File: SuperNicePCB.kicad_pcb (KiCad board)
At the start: 4 copper layers, 75 x 85 mm, 66 parts, among them U1 ESP32-S3-WROOM-1-N8, U2 SY8089AAAC, U3 SGM2048-ADJXTEK8G/TR, U4 ICS-43434_C5656610, U5 AM312, U6 SCD40-D-R1, U7 SHT40-AD1B-R3, U8 HLK-LD6002, U9 DWM3000TR13

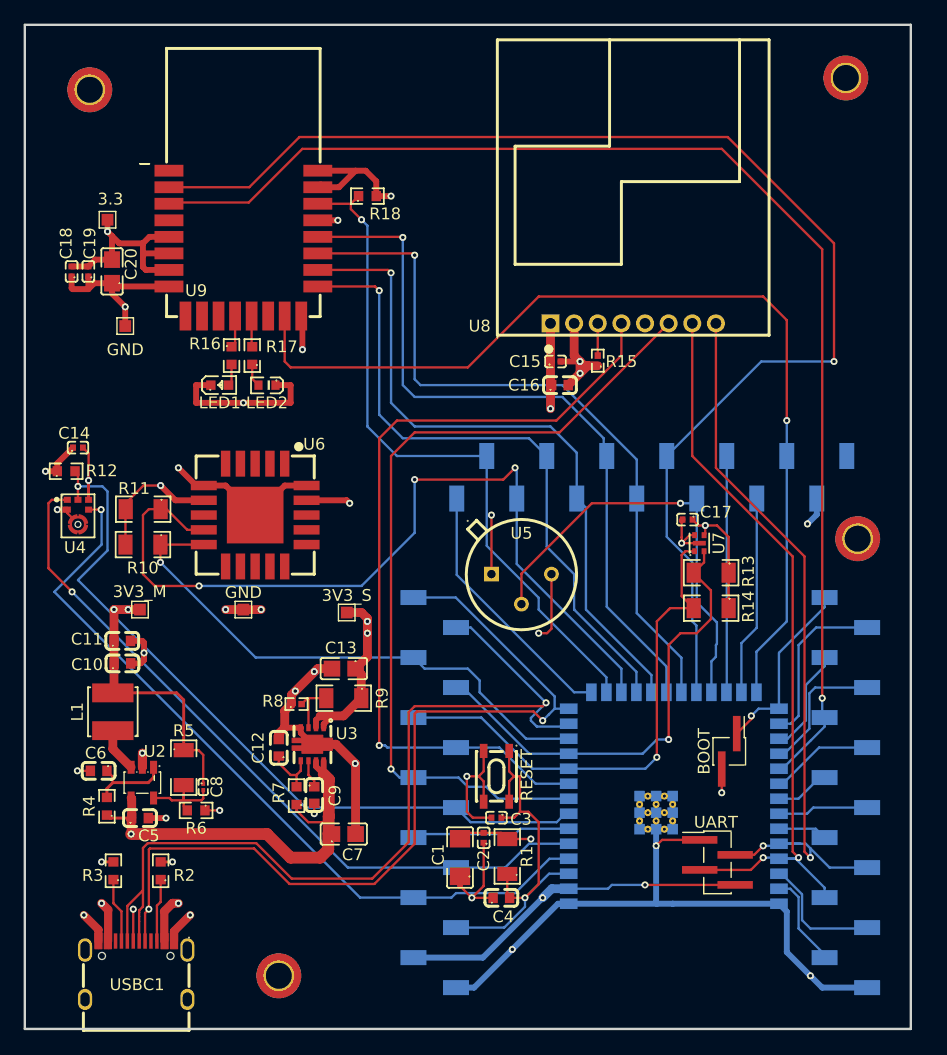
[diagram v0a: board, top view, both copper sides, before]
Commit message: Label + test commit Mathieu
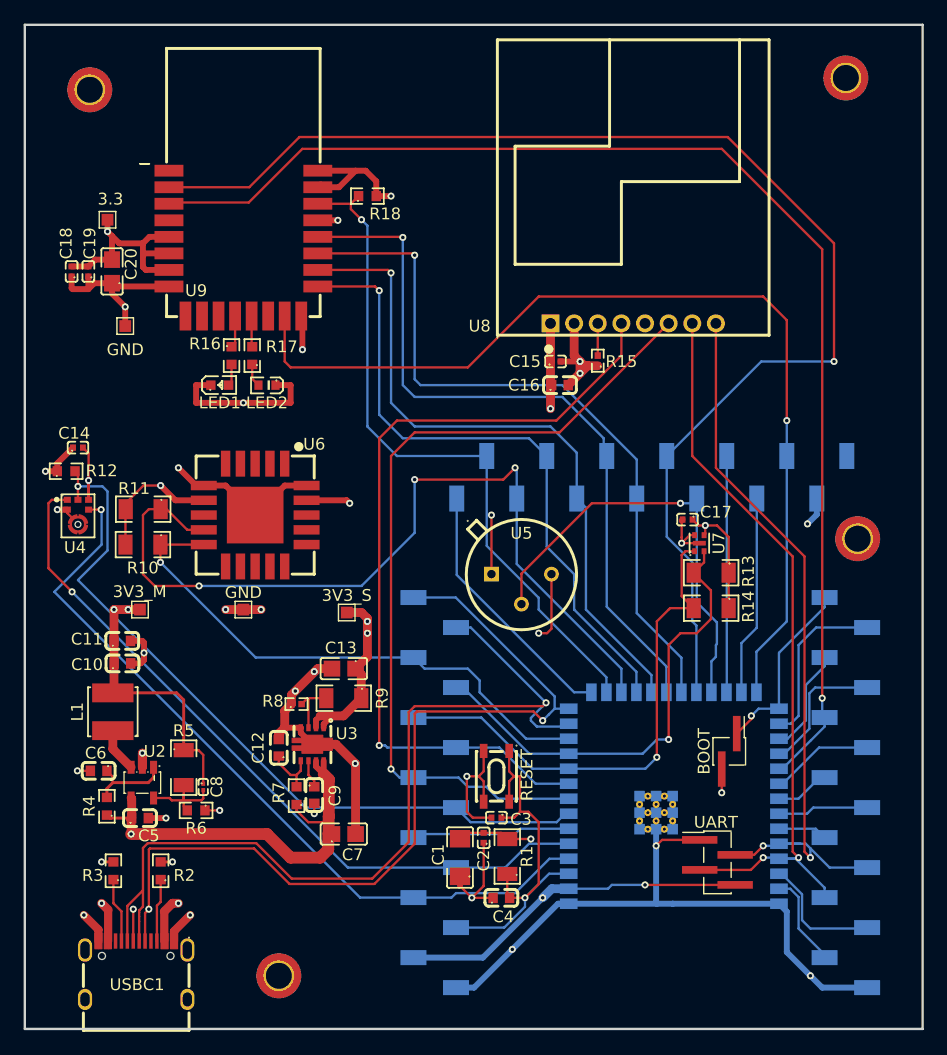
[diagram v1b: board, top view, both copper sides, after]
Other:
- board size 75 x 85 mm -> 76 x 85 mm
- board text added: "BOOT"
- board text added: "GND"
- board text added: "IO1"
- board text added: "IO2"
- board text added: "IO35"
- board text added: "IO36"
- board text added: "IO37"
- board text added: "IO39"
- board text added: "IO40"
- board text added: "IO41"
- board text added: "IO42"
- board text added: "RXD"
- board text added: "TXD"
- board text added: "UWB_RST"
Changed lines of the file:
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@@
 		(at 151 131.49 90)
 		(property "Reference" "H3"
-			(at 0.99 2.5 90)
+			(at 1.49 0 90)
 			(layer "B.SilkS")
 			(effects
@@
 	(gr_rect
 		(start 81.5 66.5)
-		(end 156.5 151.5)
+		(end 157.5 151.5)
 		(radius 2)
 		(stroke
@@
 		(layer "Edge.Cuts")
 	)
+	(gr_text "UWB_RST"
+		(at 152.5 125 180)
+		(layer "B.SilkS")
+		(effects
+			(font
+				(size 0.7 0.7)
+				(thickness 0.1)
+			)
+			(justify left bottom mirror)
+		)
+	)
+	(gr_text "BOOT"
+		(at 154.5 114.5 180)
+		(layer "B.SilkS")
+		(effects
+			(font
+				(size 0.7 0.7)
+				(thickness 0.1)
+			)
+			(justify left bottom mirror)
+		)
+	)
+	(gr_text "IO35"
+		(at 154.5 117 180)
+		(layer "B.SilkS")
+		(effects
+			(font
+				(size 0.7 0.7)
+				(thickness 0.1)
+			)
+			(justify left bottom mirror)
+		)
+	)
+	(gr_text "IO36"
+		(at 154.5 120 180)
+		(layer "B.SilkS")
+		(effects
+			(font
+				(size 0.7 0.7)
+				(thickness 0.1)
+			)
+			(justify left bottom mirror)
+		)
+	)
+	(gr_text "IO37"
+		(at 154.5 122.5 180)
+		(layer "B.SilkS")
+		(effects
+			(font
+				(size 0.7 0.7)
+				(thickness 0.1)
+			)
+			(justify left bottom mirror)
+		)
+	)
+	(gr_text "IO39"
+		(at 154.5 127.5 180)
+		(layer "B.SilkS")
+		(effects
+			(font
+				(size 0.7 0.7)
+				(thickness 0.1)
+			)
+			(justify left bottom mirror)
+		)
+	)
+	(gr_text "IO40"
+		(at 154.5 130 180)
+		(layer "B.SilkS")
+		(effects
+			(font
+				(size 0.7 0.7)
+				(thickness 0.1)
+			)
+			(justify left bottom mirror)
+		)
+	)
+	(gr_text "IO41"
+		(at 154.5 132.5 180)
+		(layer "B.SilkS")
+		(effects
+			(font
+				(size 0.7 0.7)
+				(thickness 0.1)
+			)
+			(justify left bottom mirror)
+		)
+	)
+	(gr_text "IO42"
+		(at 154.5 135 180)
+		(layer "B.SilkS")
+		(effects
+			(font
+				(size 0.7 0.7)
+				(thickness 0.1)
+			)
+			(justify left bottom mirror)
+		)
+	)
+	(gr_text "RXD"
+		(at 154.5 137.5 180)
+		(layer "B.SilkS")
+		(effects
+			(font
+				(size 0.7 0.7)
+				(thickness 0.1)
+			)
+			(justify left bottom mirror)
+		)
+	)
+	(gr_text "TXD"
+		(at 154.5 140 180)
+		(layer "B.SilkS")
+		(effects
+			(font
+				(size 0.7 0.7)
+				(thickness 0.1)
+			)
+			(justify left bottom mirror)
+		)
+	)
+	(gr_text "IO2"
+		(at 154.5 142.5 180)
+		(layer "B.SilkS")
+		(effects
+			(font
+				(size 0.7 0.7)
+				(thickness 0.1)
+			)
+			(justify left bottom mirror)
+		)
+	)
+	(gr_text "IO1"
+		(at 154.5 145 180)
+		(layer "B.SilkS")
+		(effects
+			(font
+				(size 0.7 0.7)
+				(thickness 0.1)
+			)
+			(justify left bottom mirror)
+		)
+	)
+	(gr_text "GND"
+		(at 154.5 147.5 180)
+		(layer "B.SilkS")
+		(effects
+			(font
+				(size 0.7 0.7)
+				(thickness 0.1)
+			)
+			(justify left bottom mirror)
+		)
+	)
 	(dimension
